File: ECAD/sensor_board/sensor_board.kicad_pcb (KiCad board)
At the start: 2 copper layers, 40.6 x 35.6 mm, 36 parts, among them J2 Conn_01x04, J4 S4B-XH-SM4-TB, Q2 Q_PMOS_GSD, Q3 Q_PMOS_GSD, Q4 2N7002, U1 TPL5111, U2 TPS22917DBV, U3 TC2030, U4 BC805M, Y1 32.768kHz

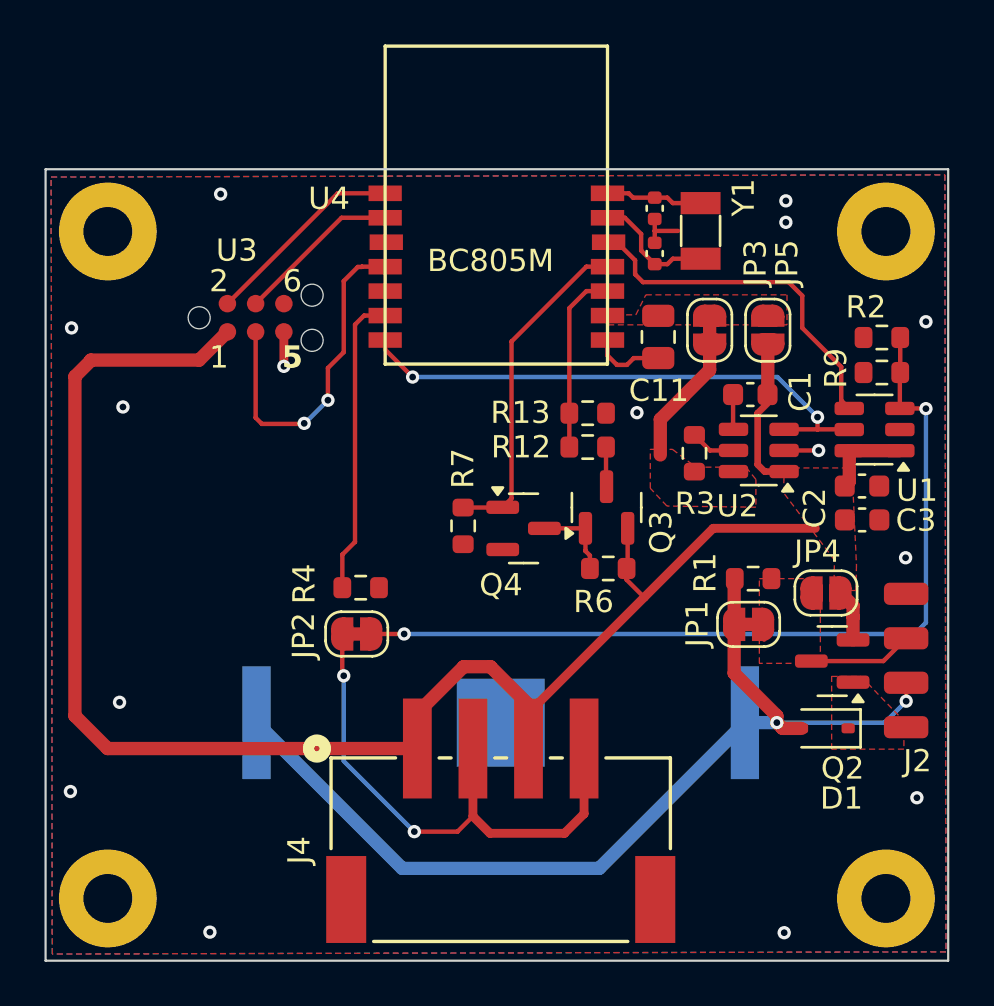
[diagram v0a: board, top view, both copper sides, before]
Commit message: Updated board layout
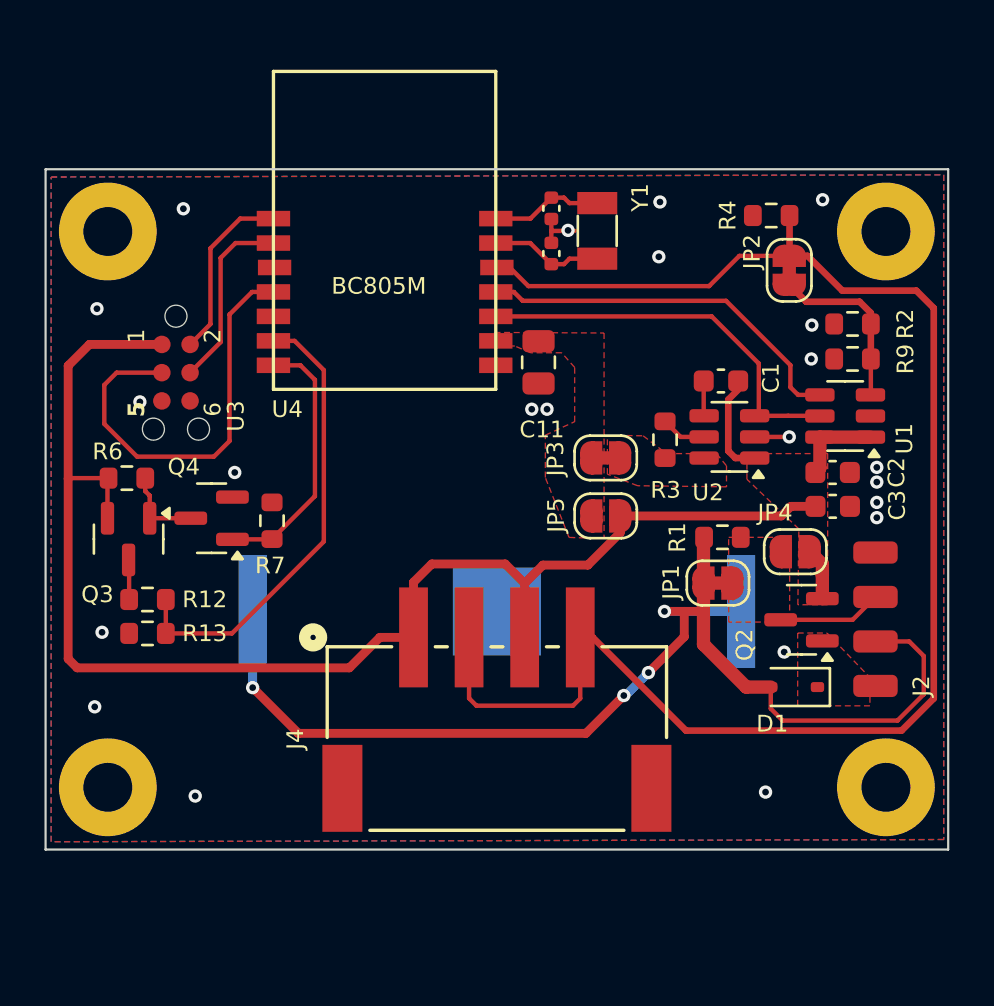
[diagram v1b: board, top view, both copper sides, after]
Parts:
- moved JP2 25.4 mm to (33.5, 4.55), turned to 90 degrees
- moved R4 24.9 mm to (32.6, 2.08), turned to 180 degrees
- moved R13 22.1 mm to (4.58, 20.9), turned to 180 degrees
- moved R6 22.0 mm to (3.66, 13.9), turned to 0 degrees
- moved Q3 21.5 mm to (3.73, 16.6), turned to -90 degrees
- moved R12 21.0 mm to (4.58, 19.4), turned to 0 degrees
- moved Q4 14.0 mm to (7.47, 15.7), turned to 180 degrees
- moved JP5 11.1 mm to (25.2, 15.6), turned to 180 degrees
- moved R7 8.60 mm to (10.2, 15.8), turned to 90 degrees
- moved JP3 7.41 mm to (25.2, 13.0), turned to 180 degrees
- moved C11 5.50 mm to (22.2, 8.69)
- moved U4 5.15 mm to (10.2, 9.90)
- moved BT2 5.00 mm to (20.3, 19.9)
- moved J4 5.00 mm to (20.3, 25.6)
- moved H3 5.00 mm to (2.80, 27.8)
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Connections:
- U4 pad 10: /BATT_DIV -> /NDRV
- U4 pad 11: /SENSE_CTRL -> /DONE_SIGNAL
- U4 pad 12: /DONE_SIGNAL -> /FLOW_SENSE
- U4 pad 6: /FLOW_SENSE -> /BATT_DIV
- U4 pad 7: /NDRV -> /SENSE_CTRL
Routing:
- net /FLOW_SENSE: track 38.4 -> 69.9 mm, vias 2 -> 0
- net Net-(JP2-A): track 39.2 -> 7.89 mm, vias 2 -> 0
- net /BATT_DIV: track 8.28 -> 20.9 mm
- net +BATT: track 83.7 -> 74.3 mm
- net Net-(D1-A2): track 44.4 -> 53.2 mm, vias 2 -> 4
- net /NDRV: track 24.6 -> 18.1 mm, vias 2 -> 0
- net PWR_GATED: track 5.88 -> 0.00 mm
- net GND: track 8.50 -> 3.67 mm, vias 15 -> 22
- net Net-(U3-NRST): track 15.5 -> 19.2 mm, vias 2 -> 0
- net /SENSE_CTRL: track 15.1 -> 11.9 mm
- net Net-(U3-SWDIO/TMS): track 9.15 -> 8.09 mm
- net /DONE_SIGNAL: track 16.0 -> 17.1 mm
- net Net-(U3-SWCLK/TCK): track 7.43 -> 8.38 mm
- net /Xb: track 4.37 -> 5.06 mm
- net /Xa: track 5.59 -> 5.06 mm
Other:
- board size 40.6 x 35.6 mm -> 40.6 x 30.6 mm
